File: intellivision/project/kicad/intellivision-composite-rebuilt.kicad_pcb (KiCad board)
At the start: 2 copper layers, 32.5 x 33.5 mm, 21 parts, among them J1 VID IN, J2 VID OUT, J3 AUD IN, J4 AUD OUT, J5 +5V IN, J6 GND IN, J7 GND OUT, Q1 2N3904, Q2 2N3904

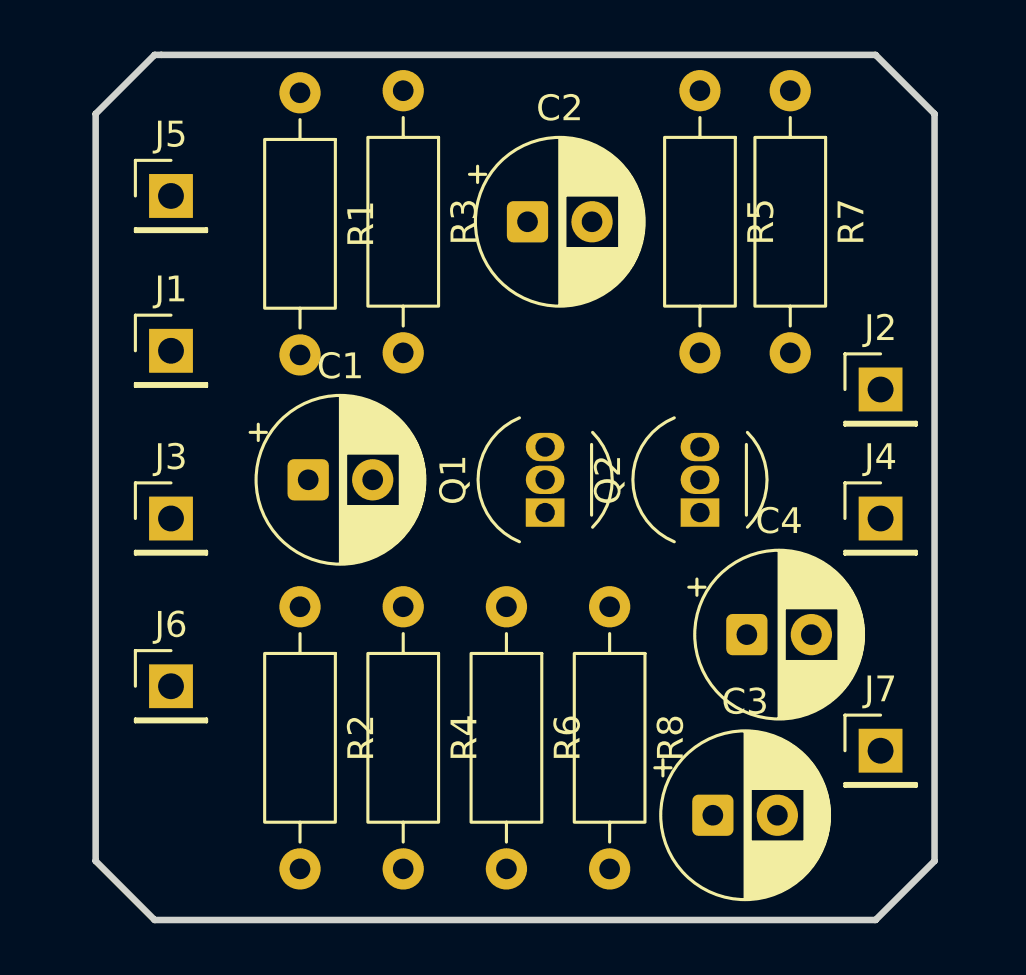
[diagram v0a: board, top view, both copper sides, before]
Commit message: Add routing
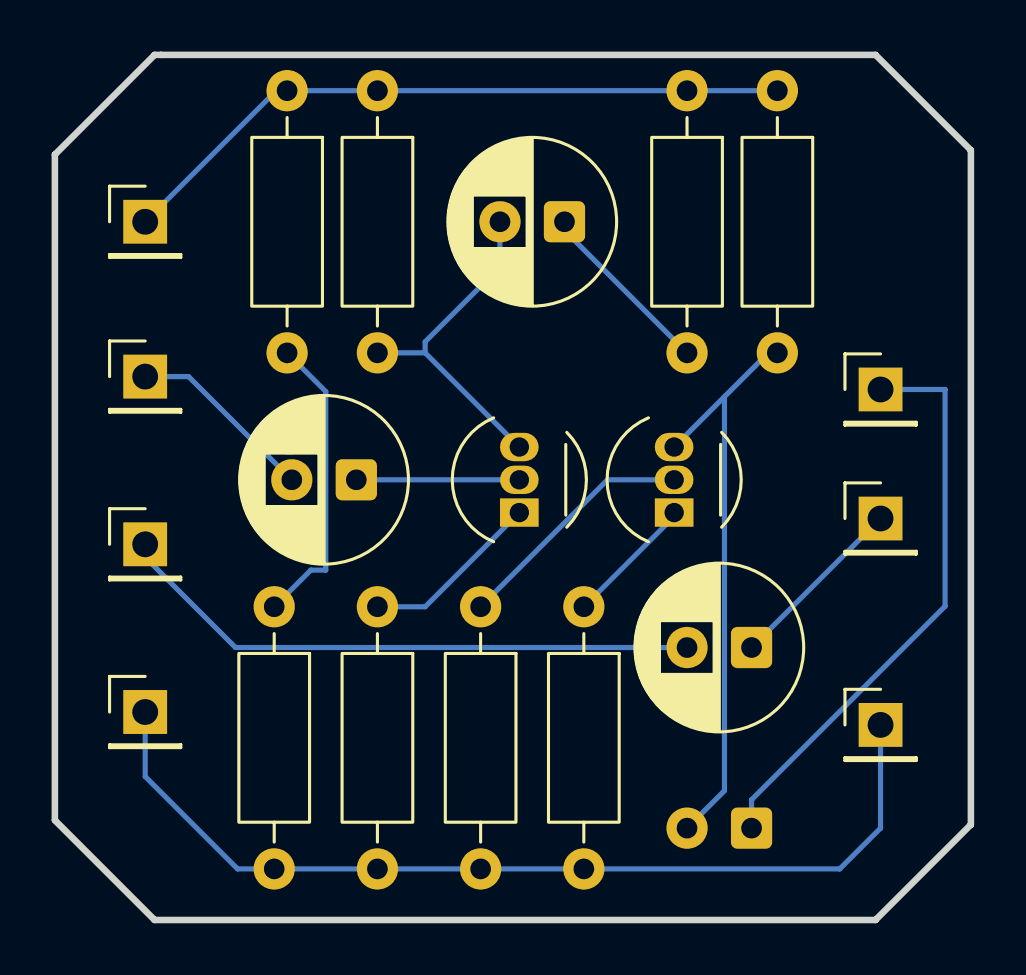
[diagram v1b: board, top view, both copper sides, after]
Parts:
- C3: moved to B.Cu
- moved C1 1.86 mm to (78.7, 82.0), turned to 180 degrees
- moved C3 1.58 mm to (94.0, 95.5), turned to 180 degrees
- moved C2 1.43 mm to (86.8, 72.0), turned to 180 degrees
- moved J1 1.41 mm to (70.5, 78.0)
- moved J3 1.41 mm to (70.5, 84.5)
- moved J5 1.41 mm to (70.5, 72.0)
- moved J6 1.41 mm to (70.5, 91.0)
- moved J7 1.00 mm to (99.0, 91.5)
- moved Q1 1.00 mm to (85.0, 83.3)
- moved Q2 1.00 mm to (91.0, 83.3)
- moved R2 1.00 mm to (75.5, 86.9)
- moved R3 1.00 mm to (79.5, 66.9)
- moved R4 1.00 mm to (79.5, 86.9)
- moved R6 1.00 mm to (83.5, 86.9)
- moved R8 1.00 mm to (87.5, 86.9)
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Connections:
- C1 pad 1: Net-(Q1-B) -> Net-(J1-Pin_1)
- C1 pad 2: Net-(J1-Pin_1) -> Net-(Q1-B)
- J6 pad 1: Net-(J6-Pin_1) -> GND
- J7 pad 1: Net-(J6-Pin_1) -> GND
- R4 pad 2: Net-(J6-Pin_1) -> GND
- R6 pad 2: Net-(J6-Pin_1) -> GND
- R8 pad 2: Net-(J6-Pin_1) -> GND
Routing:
- net GND: track 0.00 -> 37.6 mm
- net +5V: track 0.00 -> 26.8 mm
- net Net-(J3-Pin_1): track 0.00 -> 22.9 mm
- net Net-(Q2-C): track 0.00 -> 22.9 mm
- net Net-(J2-Pin_1): track 0.00 -> 22.6 mm
- net Net-(Q2-B): track 0.00 -> 16.6 mm
- net Net-(Q1-C): track 0.00 -> 13.3 mm
- net Net-(R1-Pad2): track 0.00 -> 11.6 mm
- net Net-(J1-Pin_1): track 0.00 -> 7.34 mm
- net Net-(J4-Pin_1): track 0.00 -> 7.07 mm
- net Net-(Q1-E): track 0.00 -> 7.01 mm
- net Net-(Q1-B): track 0.00 -> 6.32 mm
- net Net-(Q2-E): track 0.00 -> 5.10 mm
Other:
- board size 32.5 x 33.5 mm -> 35.5 x 33.5 mm
